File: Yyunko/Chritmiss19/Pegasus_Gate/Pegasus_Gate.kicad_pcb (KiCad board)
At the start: 2 copper layers, 68.2 x 67.6 mm, 37 parts, among them J1 Conn_01x03_Female, J2 Conn_01x03_Female, U1 WS2811, U2 WS2811, U3 WS2811, U4 WS2811

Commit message: Begin work on assigning part nums
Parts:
- DA1, DA2, DA3: value WS2812B -> BL-HRGB32K-3-TRBCT-ND
- DB1, DB10, DB11, DB12, DB2, DB3, DB4, DB5, DB6, DB7, DB8, DB9: value LED -> 754-1437-6-ND
- DC1, DC2, DC3, DC4, DD1, DD2, DD3: value WS2812B -> 1830-1206-1-ND
- U4: value WS2811 -> 1528-1537-ND
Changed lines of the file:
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@@
       (effects (font (size 1 1) (thickness 0.15)) (justify mirror))
     )
-    (fp_text value WS2812B (at -3.556 -6.604 260) (layer B.Fab)
+    (fp_text value 1830-1206-1-ND (at -3.556 -6.604 260) (layer B.Fab)
       (effects (font (size 1 1) (thickness 0.15)) (justify mirror))
     )
@@
       (effects (font (size 1 1) (thickness 0.15)) (justify mirror))
     )
-    (fp_text value WS2812B (at -3.556 -6.604 220) (layer B.Fab)
+    (fp_text value 1830-1206-1-ND (at -3.556 -6.604 220) (layer B.Fab)
       (effects (font (size 1 1) (thickness 0.15)) (justify mirror))
     )
@@
       (effects (font (size 1 1) (thickness 0.15)) (justify mirror))
     )
-    (fp_text value WS2812B (at -3.556 -6.604 180) (layer B.Fab)
+    (fp_text value 1830-1206-1-ND (at -3.556 -6.604 180) (layer B.Fab)
       (effects (font (size 1 1) (thickness 0.15)) (justify mirror))
     )
@@
       (effects (font (size 1 1) (thickness 0.15)) (justify mirror))
     )
-    (fp_text value WS2812B (at -3.556 -6.604 90) (layer B.Fab)
+    (fp_text value 1830-1206-1-ND (at -3.556 -6.604 90) (layer B.Fab)
       (effects (font (size 1 1) (thickness 0.15)) (justify mirror))
     )
@@
       (effects (font (size 1 1) (thickness 0.15)) (justify mirror))
     )
-    (fp_text value WS2812B (at -3.556 -6.604 60) (layer B.Fab)
+    (fp_text value 1830-1206-1-ND (at -3.556 -6.604 60) (layer B.Fab)
       (effects (font (size 1 1) (thickness 0.15)) (justify mirror))
     )
@@
       (effects (font (size 1 1) (thickness 0.15)) (justify mirror))
     )
-    (fp_text value WS2812B (at -3.556 -6.604 30) (layer B.Fab)
+    (fp_text value 1830-1206-1-ND (at -3.556 -6.604 30) (layer B.Fab)
       (effects (font (size 1 1) (thickness 0.15)) (justify mirror))
     )
@@
       (effects (font (size 1 1) (thickness 0.15)) (justify mirror))
     )
-    (fp_text value WS2812B (at -3.556 -6.604) (layer B.Fab)
+    (fp_text value 1830-1206-1-ND (at -3.556 -6.604) (layer B.Fab)
       (effects (font (size 1 1) (thickness 0.15)) (justify mirror))
     )
@@
       (effects (font (size 1 1) (thickness 0.15)) (justify mirror))
     )
-    (fp_text value WS2811 (at 0 -3.75 90) (layer B.Fab)
+    (fp_text value 1528-1537-ND (at 0 -3.75 90) (layer B.Fab)
       (effects (font (size 1 1) (thickness 0.15)) (justify mirror))
     )
@@
       (effects (font (size 1 1) (thickness 0.15)))
     )
-    (fp_text value WS2812B (at 0 4 80) (layer F.Fab)
+    (fp_text value BL-HRGB32K-3-TRBCT-ND (at 0 4 80) (layer F.Fab)
       (effects (font (size 1 1) (thickness 0.15)))
     )
@@
       (effects (font (size 1 1) (thickness 0.15)))
     )
-    (fp_text value WS2812B (at 0 4 40) (layer F.Fab)
+    (fp_text value BL-HRGB32K-3-TRBCT-ND (at 0 4 40) (layer F.Fab)
       (effects (font (size 1 1) (thickness 0.15)))
     )
@@
       (effects (font (size 1 1) (thickness 0.15)))
     )
-    (fp_text value LED (at 0 1.6 260) (layer F.Fab)
+    (fp_text value 754-1437-6-ND (at 0 1.6 260) (layer F.Fab)
       (effects (font (size 1 1) (thickness 0.15)))
     )
@@
       (effects (font (size 1 1) (thickness 0.15)))
     )
-    (fp_text value LED (at 0 1.6 10) (layer F.Fab)
+    (fp_text value 754-1437-6-ND (at 0 1.6 10) (layer F.Fab)
       (effects (font (size 1 1) (thickness 0.15)))
     )
@@
       (effects (font (size 1 1) (thickness 0.15)))
     )
-    (fp_text value LED (at 0 1.6) (layer F.Fab)
+    (fp_text value 754-1437-6-ND (at 0 1.6) (layer F.Fab)
       (effects (font (size 1 1) (thickness 0.15)))
     )
@@
       (effects (font (size 1 1) (thickness 0.15)))
     )
-    (fp_text value LED (at 0 1.6 350) (layer F.Fab)
+    (fp_text value 754-1437-6-ND (at 0 1.6 350) (layer F.Fab)
       (effects (font (size 1 1) (thickness 0.15)))
     )
@@
       (effects (font (size 1 1) (thickness 0.15)))
     )
-    (fp_text value LED (at 0 1.6 340) (layer F.Fab)
+    (fp_text value 754-1437-6-ND (at 0 1.6 340) (layer F.Fab)
       (effects (font (size 1 1) (thickness 0.15)))
     )
@@
       (effects (font (size 1 1) (thickness 0.15)))
     )
-    (fp_text value LED (at 0 1.6 330) (layer F.Fab)
+    (fp_text value 754-1437-6-ND (at 0 1.6 330) (layer F.Fab)
       (effects (font (size 1 1) (thickness 0.15)))
     )
@@
       (effects (font (size 1 1) (thickness 0.15)))
     )
-    (fp_text value LED (at 0 1.6 320) (layer F.Fab)
+    (fp_text value 754-1437-6-ND (at 0 1.6 320) (layer F.Fab)
       (effects (font (size 1 1) (thickness 0.15)))
     )
@@
       (effects (font (size 1 1) (thickness 0.15)))
     )
-    (fp_text value LED (at 0 1.6 310) (layer F.Fab)
+    (fp_text value 754-1437-6-ND (at 0 1.6 310) (layer F.Fab)
       (effects (font (size 1 1) (thickness 0.15)))
     )
@@
       (effects (font (size 1 1) (thickness 0.15)))
     )
-    (fp_text value LED (at 0 1.6 300) (layer F.Fab)
+    (fp_text value 754-1437-6-ND (at 0 1.6 300) (layer F.Fab)
       (effects (font (size 1 1) (thickness 0.15)))
     )
@@
       (effects (font (size 1 1) (thickness 0.15)))
     )
-    (fp_text value LED (at 0 1.6 290) (layer F.Fab)
+    (fp_text value 754-1437-6-ND (at 0 1.6 290) (layer F.Fab)
       (effects (font (size 1 1) (thickness 0.15)))
     )
@@
       (effects (font (size 1 1) (thickness 0.15)))
     )
-    (fp_text value LED (at 0 1.6 280) (layer F.Fab)
+    (fp_text value 754-1437-6-ND (at 0 1.6 280) (layer F.Fab)
       (effects (font (size 1 1) (thickness 0.15)))
     )
@@
       (effects (font (size 1 1) (thickness 0.15)))
     )
-    (fp_text value LED (at 0 1.6 270) (layer F.Fab)
+    (fp_text value 754-1437-6-ND (at 0 1.6 270) (layer F.Fab)
       (effects (font (size 1 1) (thickness 0.15)))
     )
@@
       (effects (font (size 1 1) (thickness 0.15)))
     )
-    (fp_text value WS2812B (at 0 4) (layer F.Fab)
+    (fp_text value BL-HRGB32K-3-TRBCT-ND (at 0 4) (layer F.Fab)
       (effects (font (size 1 1) (thickness 0.15)))
     )
@@
   (segment (start 148.0146 71.9494) (end 153.5938 71.9494) (width 0.25) (layer F.Cu) (net 3))
   (segment (start 143.002 76.962) (end 148.0146 71.9494) (width 0.25) (layer F.Cu) (net 3))
-  (via (at 123.952 81.28) (size 0.8) (drill 0.4) (layers F.Cu B.Cu) (net 29))
-  (via (at 157.226 70.739) (size 0.8) (drill 0.4) (layers F.Cu B.Cu) (net 29))
-  (via (at 105.41 110.109) (size 0.8) (drill 0.4) (layers F.Cu B.Cu) (net 29))
   (segment (start 111.58286 104.895097) (end 111.58286 102.28514) (width 0.25) (layer F.Cu) (net 5))
   (segment (start 111.005017 105.47294) (end 111.58286 104.895097) (width 0.25) (layer F.Cu) (net 5))
@@
   (segment (start 136.89067 82.296) (end 134.582315 84.604355) (width 0.25) (layer B.Cu) (net 28))
   (segment (start 140.081 82.296) (end 136.89067 82.296) (width 0.25) (layer B.Cu) (net 28))
+  (via (at 123.952 81.28) (size 0.8) (drill 0.4) (layers F.Cu B.Cu) (net 29))
+  (via (at 157.226 70.739) (size 0.8) (drill 0.4) (layers F.Cu B.Cu) (net 29))
+  (via (at 105.41 110.109) (size 0.8) (drill 0.4) (layers F.Cu B.Cu) (net 29))
   (segment (start 101.222859 110.473013) (end 100.673361 111.022511) (width 0.25) (layer B.Cu) (net 29))
   (segment (start 100.673361 111.022511) (end 100.457 112.249554) (width 0.25) (layer B.Cu) (net 29))

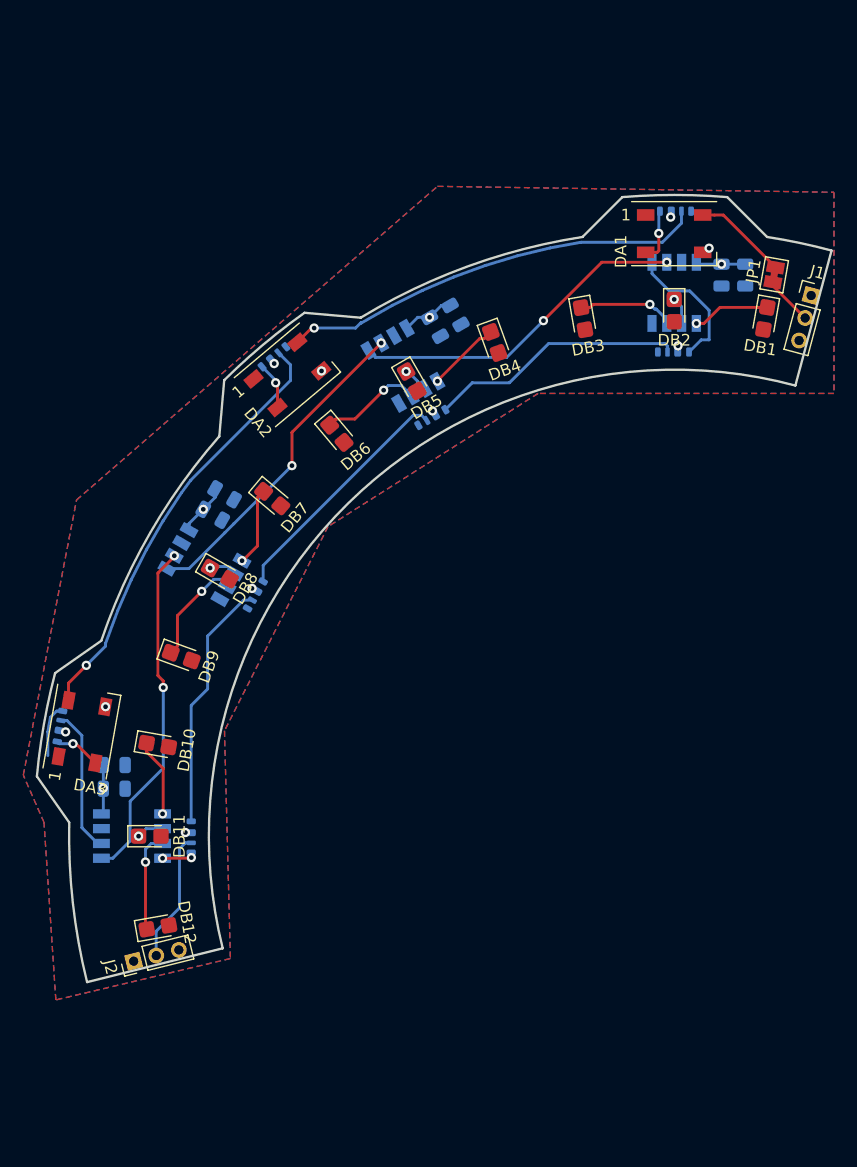
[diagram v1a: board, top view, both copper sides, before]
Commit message: Continue work on durg ring thing
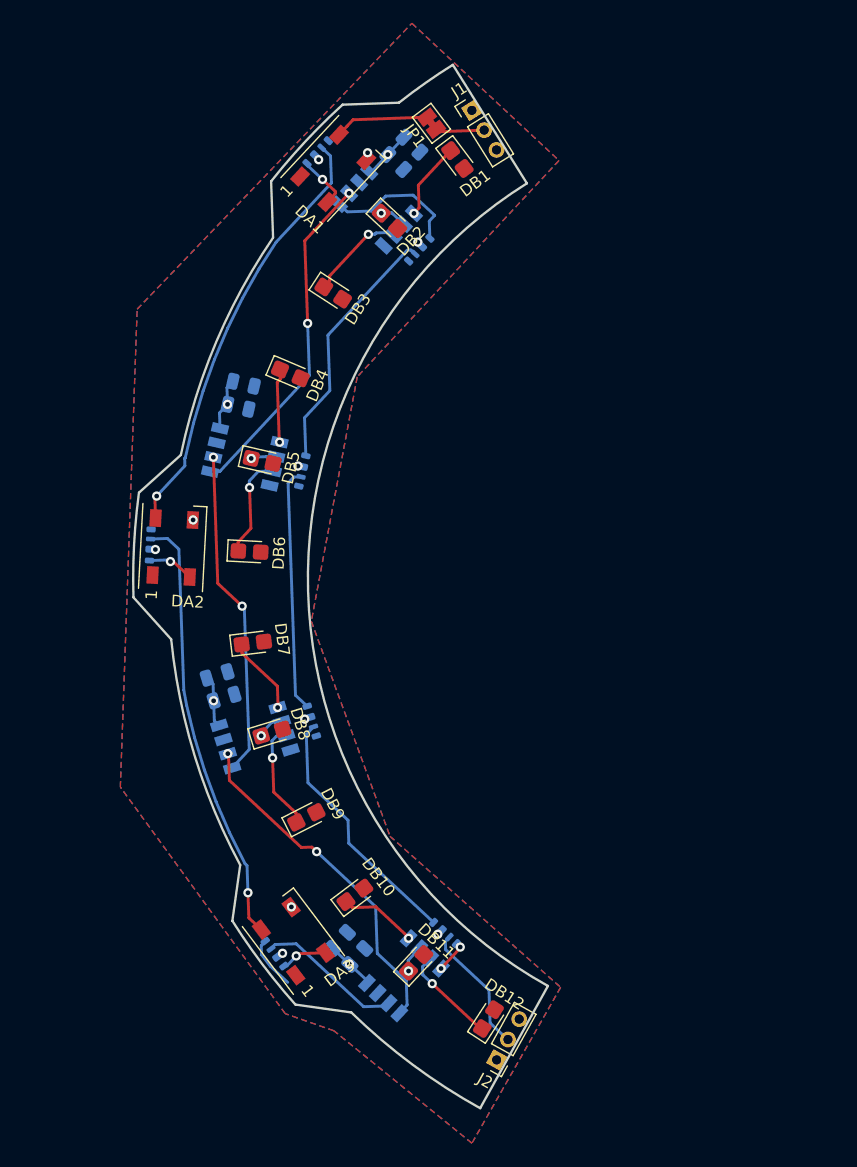
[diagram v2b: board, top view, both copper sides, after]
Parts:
- added SYM1: SYM_Radioactive_Large, Local:DragonIcon, B.Cu at (117.2, 99.4)
- moved J1 33.2 mm to (136.9, 58.9), turned to 32 degrees
- moved J2 32.3 mm to (139.0, 140.4), turned to 151 degrees
- moved JP1 32.2 mm to (133.4, 60.0), turned to 127 degrees
- moved DD1 31.1 mm to (123.6, 62.5), turned to 227 degrees
- moved C1 30.7 mm to (131.7, 61.9), turned to 317 degrees
- moved DA1 29.8 mm to (125.0, 63.9), turned to 47 degrees
- moved DB1 29.8 mm to (135.6, 63.1), turned to 307 degrees
- moved C2 29.6 mm to (130.3, 63.3), turned to 317 degrees
- moved DB12 29.4 mm to (138.3, 136.9), turned to 57 degrees
- moved DD3 26.9 mm to (120.0, 131.4), turned to 307 degrees
- moved U4 26.6 mm to (128.7, 67.4), turned to 137 degrees
- moved U1 26.3 mm to (131.0, 133.2), turned to 227 degrees
- moved DB2 25.6 mm to (129.8, 68.4), turned to 317 degrees
- moved DA3 25.6 mm to (121.5, 130.2), turned to 127 degrees
- moved C8 25.3 mm to (127.0, 131.5), turned to 47 degrees
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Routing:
- net +5V: track 19.1 -> 21.2 mm
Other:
- board size 68.2 x 67.6 mm -> 35.6 x 89.6 mm
- board text added: "GND SIG +5V"
